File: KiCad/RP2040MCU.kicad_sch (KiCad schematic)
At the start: 49 parts, among them J6 2.54mm header 01x20, J7 2.54mm header 01x20, J8 TSA343G00-250J2, J9 C145960, Q1 SI2301B, U3 SOT-23-5 5.5V 3.3V 500mA, U4 RP2040, Y1 3225_4P

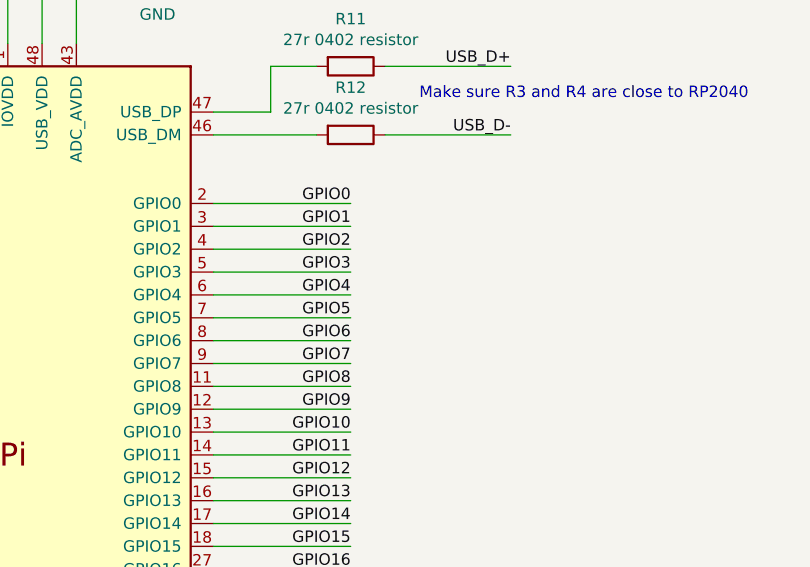
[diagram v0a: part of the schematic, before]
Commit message: I dont even remember what I changed.
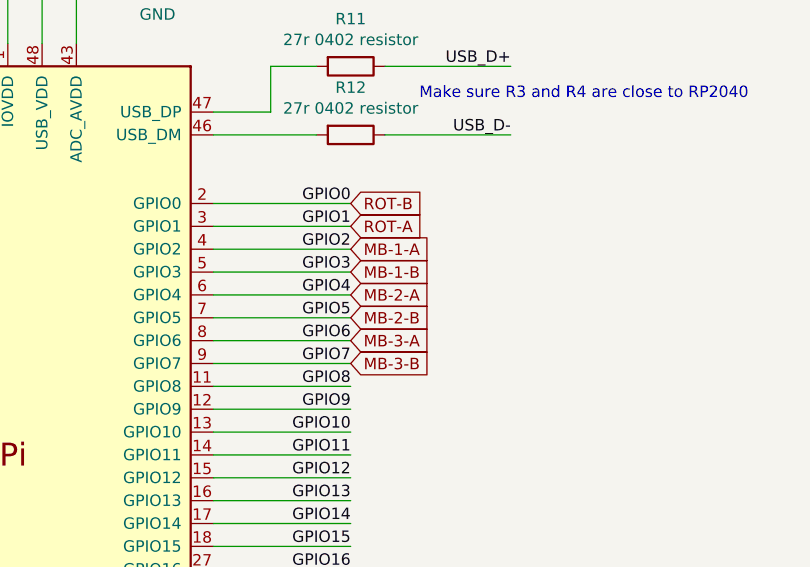
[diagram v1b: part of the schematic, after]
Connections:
- net GPIO0 renamed ROT-B
- net GPIO1 renamed ROT-A
- net GPIO2 renamed MB-1-A
- net GPIO3 renamed MB-1-B
- net GPIO4 renamed MB-2-A
- net GPIO5 renamed MB-2-B
- net GPIO6 renamed MB-3-A
- net GPIO7 renamed MB-3-B
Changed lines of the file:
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@@
+    )
+  )
+  (global_label "MB-1-A" (shape input) (at 245.11 116.84 0) (fields_autoplaced)
+    (effects (font (size 1.27 1.27)) (justify left))
+    (property "Intersheet References" "${INTERSHEET_REFS}" (id 0) (at 255.8779 116.7606 0)
+      (effects (font (size 1.27 1.27)) (justify left) hide)
+    )
+  )
+  (global_label "MB-3-A" (shape input) (at 245.11 127 0) (fields_autoplaced)
+    (effects (font (size 1.27 1.27)) (justify left))
+    (property "Intersheet References" "${INTERSHEET_REFS}" (id 0) (at 255.8779 126.9206 0)
+      (effects (font (size 1.27 1.27)) (justify left) hide)
     )
   )
@@
     )
   )
+  (global_label "ROT-A" (shape input) (at 245.11 114.3 0) (fields_autoplaced)
+    (effects (font (size 1.27 1.27)) (justify left))
+    (property "Intersheet References" "${INTERSHEET_REFS}" (id 0) (at 253.9426 114.3794 0)
+      (effects (font (size 1.27 1.27)) (justify left) hide)
+    )
+  )
   (global_label "VSYS" (shape input) (at 66.04 44.45 0) (fields_autoplaced)
     (effects (font (size 0.508 0.508)) (justify left))
     (property "Intersheet References" "${INTERSHEET_REFS}" (id 0) (at 0 0 0)
       (effects (font (size 1.27 1.27)) hide)
+    )
+  )
+  (global_label "MB-3-B" (shape input) (at 245.11 129.54 0) (fields_autoplaced)
+    (effects (font (size 1.27 1.27)) (justify left))
+    (property "Intersheet References" "${INTERSHEET_REFS}" (id 0) (at 256.0593 129.4606 0)
+      (effects (font (size 1.27 1.27)) (justify left) hide)
     )
   )
@@
     )
   )
+  (global_label "MB-2-A" (shape input) (at 245.11 121.92 0) (fields_autoplaced)
+    (effects (font (size 1.27 1.27)) (justify left))
+    (property "Intersheet References" "${INTERSHEET_REFS}" (id 0) (at 255.8779 121.8406 0)
+      (effects (font (size 1.27 1.27)) (justify left) hide)
+    )
+  )
   (global_label "VBUS" (shape input) (at 71.12 54.61 180) (fields_autoplaced)
     (effects (font (size 1.1938 1.1938)) (justify right))
@@
     )
   )
+  (global_label "ROT-B" (shape input) (at 245.11 111.76 0) (fields_autoplaced)
+    (effects (font (size 1.27 1.27)) (justify left))
+    (property "Intersheet References" "${INTERSHEET_REFS}" (id 0) (at 254.1241 111.8394 0)
+      (effects (font (size 1.27 1.27)) (justify left) hide)
+    )
+  )
   (global_label "XOUT" (shape input) (at 165.1 152.4 180) (fields_autoplaced)
     (effects (font (size 1.27 1.27)) (justify right))
@@
     )
   )
+  (global_label "MB-1-B" (shape input) (at 245.11 119.38 0) (fields_autoplaced)
+    (effects (font (size 1.27 1.27)) (justify left))
+    (property "Intersheet References" "${INTERSHEET_REFS}" (id 0) (at 256.0593 119.3006 0)
+      (effects (font (size 1.27 1.27)) (justify left) hide)
+    )
+  )
+  (global_label "MB-2-B" (shape input) (at 245.11 124.46 0) (fields_autoplaced)
+    (effects (font (size 1.27 1.27)) (justify left))
+    (property "Intersheet References" "${INTERSHEET_REFS}" (id 0) (at 256.0593 124.3806 0)
+      (effects (font (size 1.27 1.27)) (justify left) hide)
+    )
+  )
